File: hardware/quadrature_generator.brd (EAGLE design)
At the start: 160 x 100 mm, 38 parts, among them IC1 74LVC1G14, IC2 74LVC74, IC3 74LVC04, IC4 74LVC04, IC5 PT7C4511, IC6 78L33

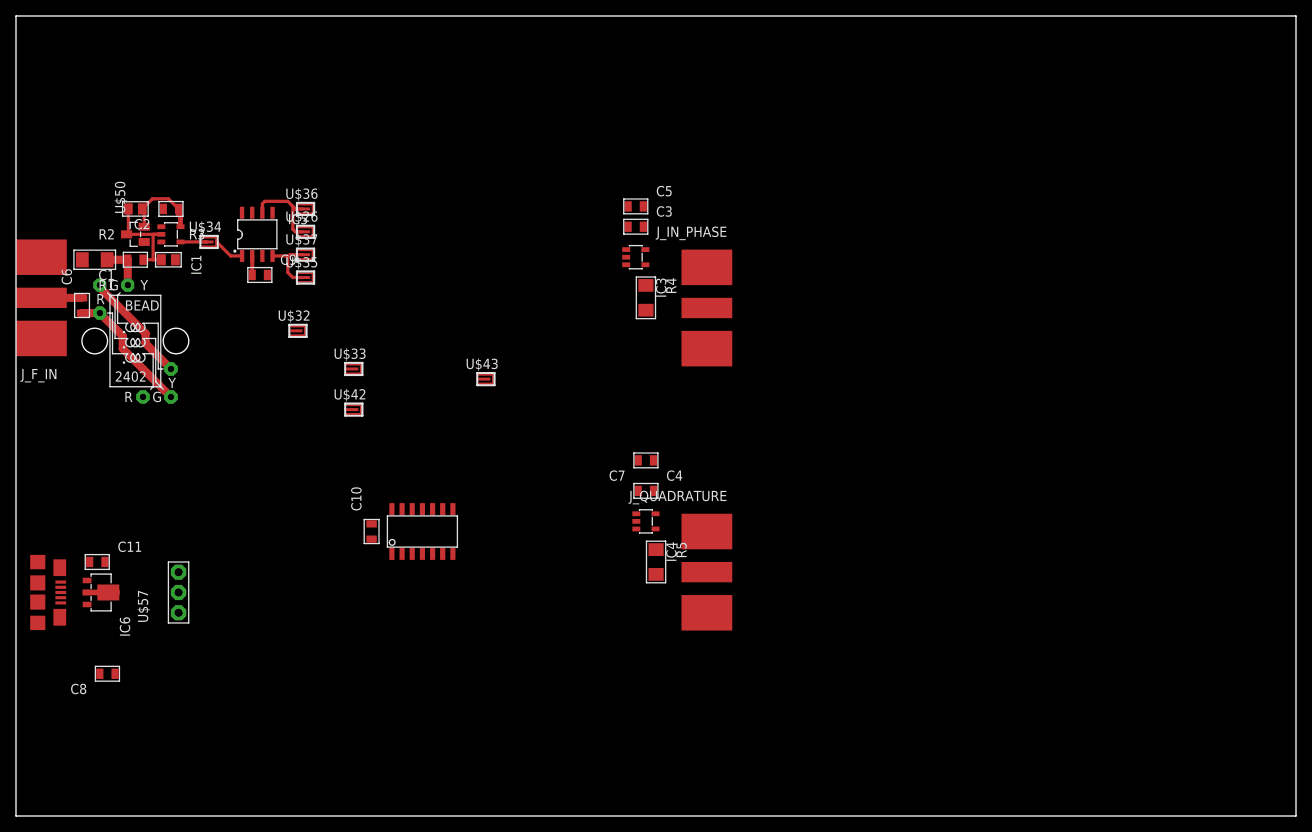
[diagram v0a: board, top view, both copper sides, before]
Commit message: checkpoint
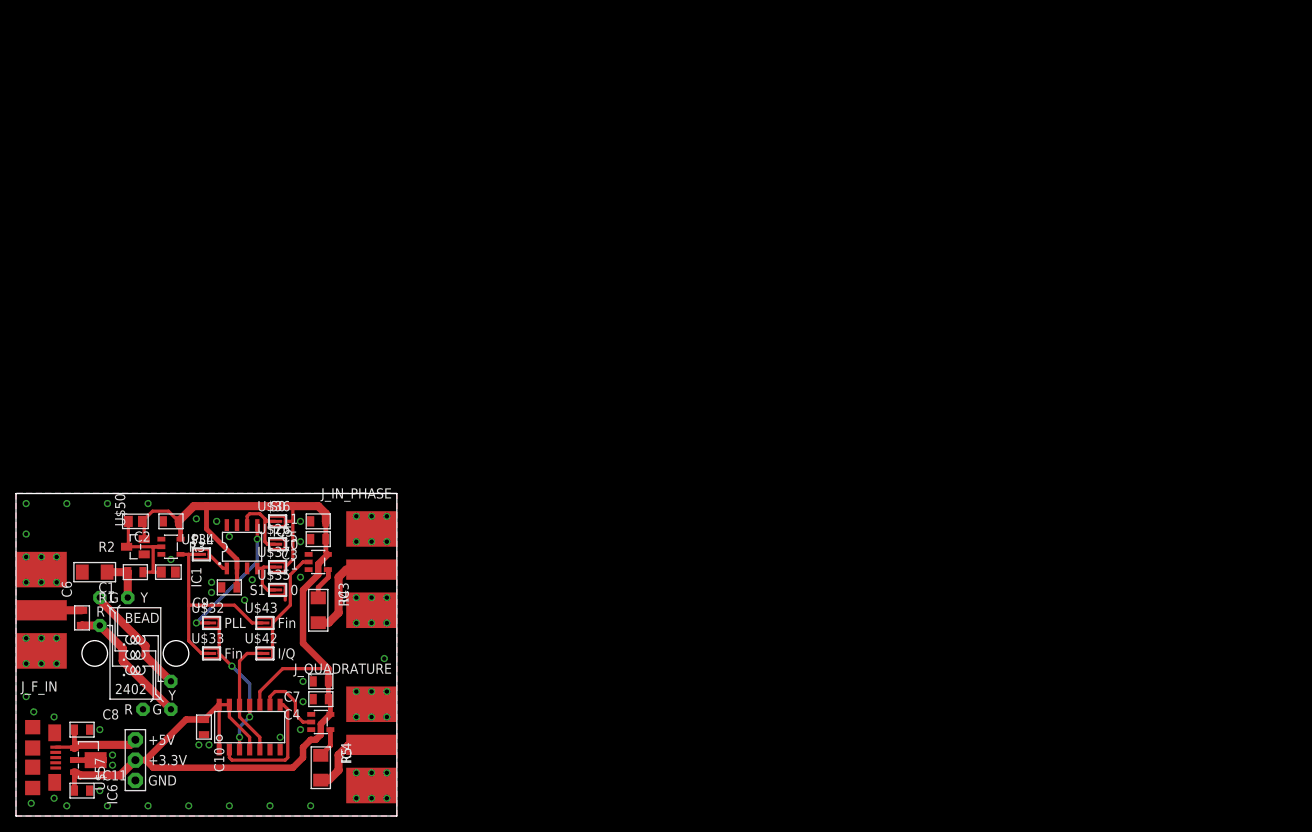
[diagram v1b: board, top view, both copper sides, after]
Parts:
- moved R4 56.6 mm to (37.8, 25.7)
- moved C5 55.9 mm to (37.8, 36.8), turned to 180 degrees
- moved C3 55.7 mm to (37.8, 34.6), turned to 180 degrees
- moved IC3 55.0 mm to (37.8, 31.8)
- moved J_IN_PHASE 53.2 mm to (44.5, 30.8)
- moved R5 49.2 mm to (38.1, 6.03)
- moved C7 49.1 mm to (38.1, 16.8)
- moved C4 48.3 mm to (38.1, 14.6), turned to 180 degrees
- moved IC4 47.8 mm to (38.1, 11.7)
- moved J_QUADRATURE 47.1 mm to (44.5, 8.89)
- moved U$43 41.1 mm to (30.8, 24.1)
- moved U$33 39.8 mm to (24.1, 20.3)
- moved C9 39.2 mm to (26.7, 28.6), turned to 180 degrees
- moved U$26 39.2 mm to (32.4, 34.0)
- moved U$37 39.2 mm to (32.4, 31.1)
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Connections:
- net +3.3V: now also U$36.2@1, U$36.2@2, U$36.2@3, U$37.2@1, U$37.2@2, U$37.2@3; no longer U$36.P$2, U$37.P$2
- net CLK_IN: now also U$33.1, U$34.1, U$43.1; no longer U$33.P$1, U$34.P$1, U$43.P$1
- net GND: now also U$26.2@1, U$26.2@2, U$26.2@3, U$35.2@1, U$35.2@2, U$35.2@3; no longer U$26.P$2, U$35.P$2
- net N$14: now also U$32.1; no longer U$32.P$1
- net N$15: now also U$34.2@1, U$34.2@2, U$34.2@3; no longer U$34.P$2
- net N$19: now also U$42.2@1, U$42.2@2, U$42.2@3, U$43.2@1, U$43.2@2, U$43.2@3; no longer U$42.P$2, U$43.P$2
- net N$7: now also U$42.1; no longer U$42.P$1
- net N$8: now also U$32.2@1, U$32.2@2, U$32.2@3, U$33.2@1, U$33.2@2, U$33.2@3; no longer U$32.P$2, U$33.P$2
- net S0: now also U$26.1, U$36.1; no longer U$26.P$1, U$36.P$1
- net S1: now also U$35.1, U$37.1; no longer U$35.P$1, U$37.P$1
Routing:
- net +3.3V: track 12.7 -> 161.8 mm
- net N$8: track 0.00 -> 25.8 mm, vias 0 -> 3
- net CLK_IN: track 3.25 -> 26.4 mm
- net N$19: track 0.00 -> 20.1 mm
- net N$14: track 0.00 -> 17.0 mm, vias 0 -> 2
- net N$9: track 0.00 -> 15.8 mm
- net N$7: track 0.00 -> 15.4 mm
- net VCC: track 0.00 -> 12.8 mm
- net N$5: track 0.00 -> 12.0 mm
- net GND: track 0.00 -> 10.8 mm, vias 0 -> 75
- net N$10: track 0.00 -> 9.29 mm
- net N$12: track 0.00 -> 8.93 mm
- net N$6: track 0.00 -> 4.09 mm
- net N$11: track 0.00 -> 3.71 mm
- net N$15: track 3.90 -> 6.12 mm
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- added copper zone on layer 1, net GND
- added copper zone on layer 16, net GND
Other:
- board size 160 x 100 mm -> 47.6 x 40.3 mm
- board text added: "+3.3V"
- board text added: "+5V"
- board text added: "0"
- board text added: "1"
- board text added: "Fin"
- board text added: "GND"
- board text added: "I/Q"
- board text added: "PLL"
- board text added: "S0"
- board text added: "S1"
